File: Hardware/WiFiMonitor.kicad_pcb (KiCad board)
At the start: 2 copper layers, 47.2 x 47.2 mm, 37 parts, among them J1 ADAP_ESP, J3 BATT, J5 FTDI, U1 4N25, U2 4N25, U3 4N25, U4 4N25, U5 MCP73831T-4ADI/OT, U6 AP1117-33, U7 DS3231MZ+

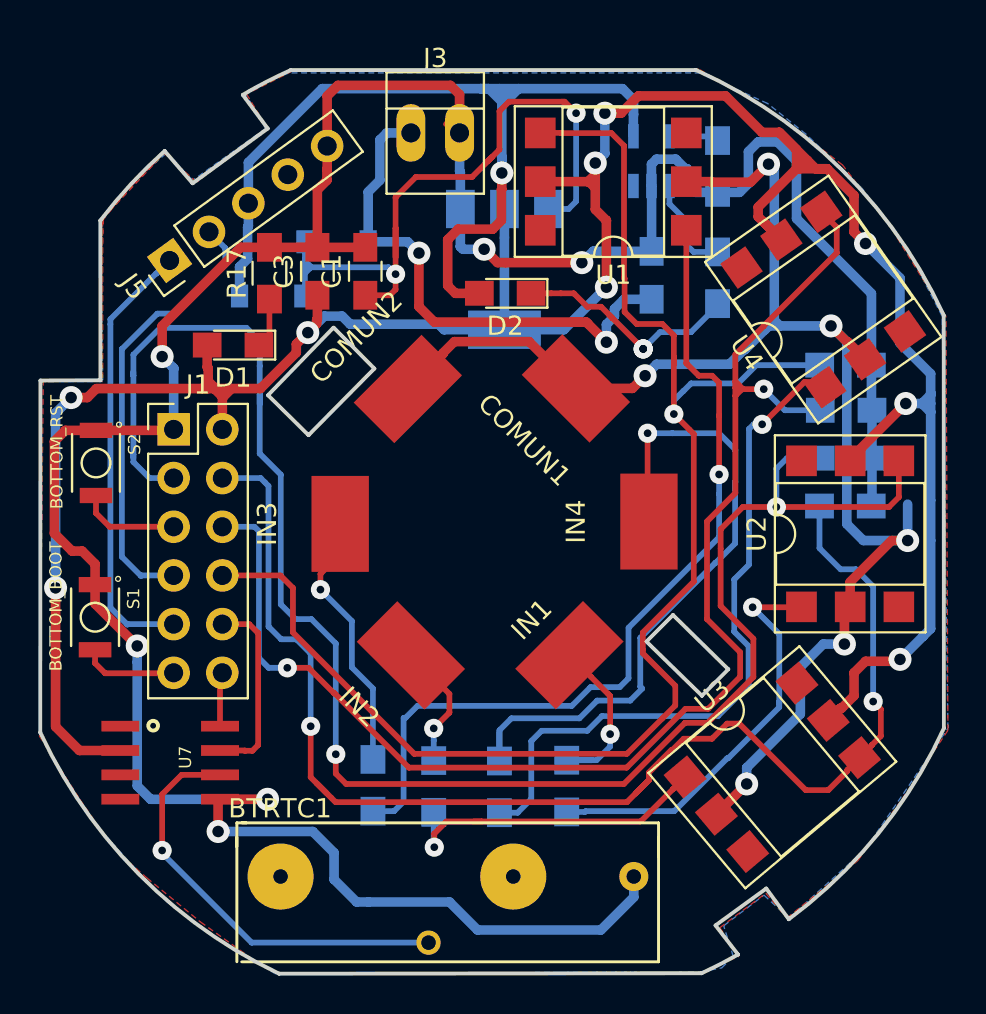
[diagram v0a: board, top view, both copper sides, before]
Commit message: PCB_PISTAS
Reacomodo de pistas
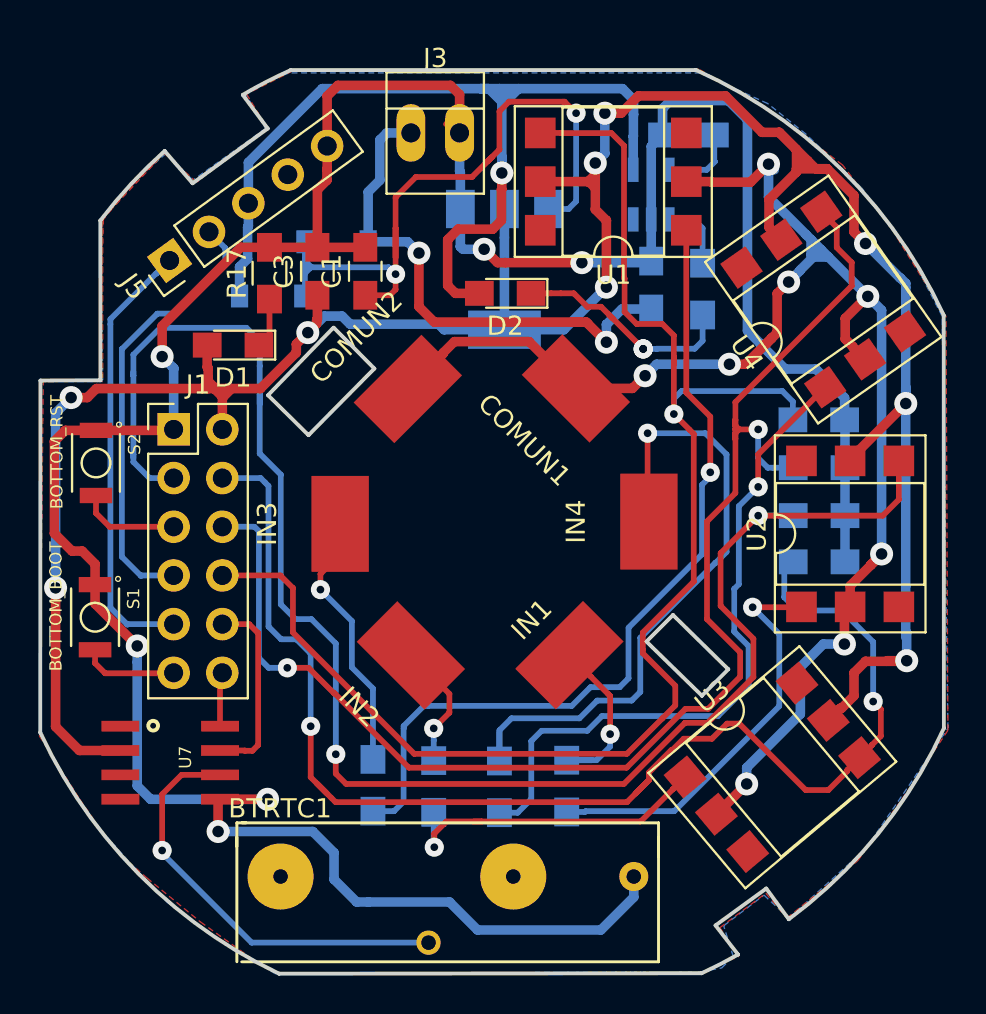
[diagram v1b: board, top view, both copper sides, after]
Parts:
- moved R6 3.31 mm to (211.7, 91.5)
- moved R8 3.31 mm to (211.7, 89.0)
- moved R7 3.22 mm to (211.7, 93.9)
- moved R5 3.18 mm to (211.7, 86.5)
- moved R14 2.24 mm to (204.9, 71.6), turned to 0 degrees
- moved U5 1.74 mm to (202.9, 74.8)
- moved R15 0.98 mm to (205.6, 79.7)
- moved C2 0.51 mm to (202.9, 79.5)
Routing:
- net GND: track 152.1 -> 155.7 mm
- net /D0: track 90.2 -> 86.9 mm
- net GNDA: track 77.6 -> 80.7 mm, vias 6 -> 8
- net +3V3: track 146.7 -> 144.2 mm
- net VCC: track 48.8 -> 50.6 mm
- net Net-(R15-Pad1): track 5.21 -> 3.76 mm
- net /D1: track 69.6 -> 68.2 mm
- net Net-(R14-Pad2): track 2.60 -> 3.96 mm
- net Net-(R3-Pad1): track 36.4 -> 35.4 mm
- net Net-(R1-Pad1): track 45.2 -> 44.2 mm
- net Net-(IN4-Pad1): track 35.6 -> 34.8 mm
- net /D2: track 77.3 -> 76.6 mm
- net /D3: track 72.4 -> 72.9 mm
